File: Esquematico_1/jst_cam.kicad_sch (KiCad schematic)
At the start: 19 parts, among them J1 Screw_Terminal_01x04, J2 Screw_Terminal_01x03, J3 Screw_Terminal_01x06, J4 Screw_Terminal_01x08, J5 SWD, J6 Screw_Terminal_01x04, J7 USB_C_Receptacle_USB2.0_16P, J8 Screw_Terminal_01x01, J9 Screw_Terminal_01x01, U5 USBLC6-2SC6

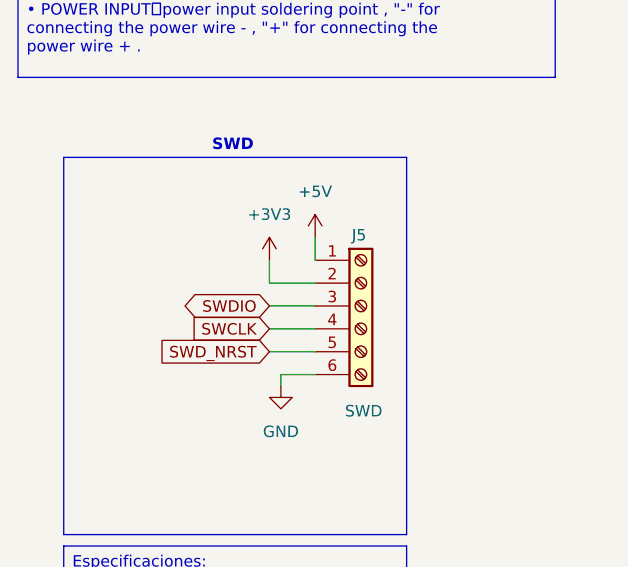
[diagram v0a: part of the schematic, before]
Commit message: Cambios de Diodos
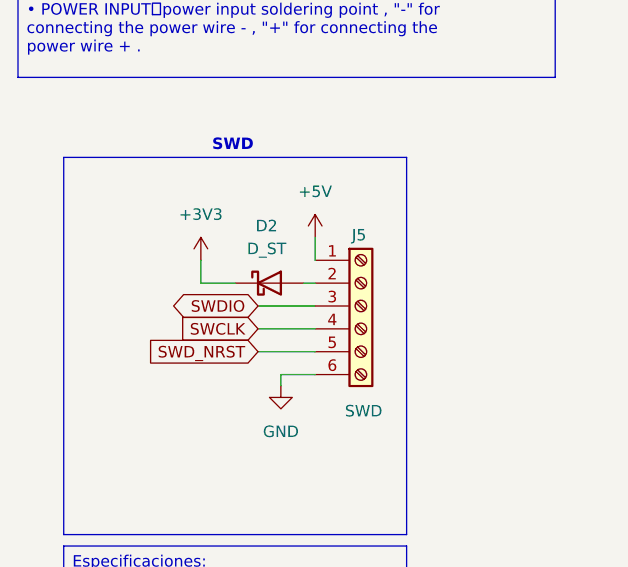
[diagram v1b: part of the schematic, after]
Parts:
- added D2: D_ST, Diode_SMD:D_SOD-323_HandSoldering, symbol Device:D_Schottky
- D3: footprint Package_TO_SOT_SMD:SOT-23 -> Diode_SMD:D_SOD-323_HandSoldering
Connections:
- net +3V3: now also D2.1 (K); no longer J5.2 (Pin_2)
- new net: D2.2 (A), J5.2 (Pin_2)
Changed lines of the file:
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@@
 	(wire
 		(pts
-			(xy 52.07 120.65) (xy 46.99 120.65)
+			(xy 45.72 45.72) (xy 49.53 45.72)
 		)
 		(stroke
@@
 	(wire
 		(pts
-			(xy 45.72 45.72) (xy 49.53 45.72)
+			(xy 63.5 40.64) (xy 68.58 40.64)
 		)
 		(stroke
@@
 	(wire
 		(pts
-			(xy 63.5 40.64) (xy 68.58 40.64)
+			(xy 130.81 133.35) (xy 130.81 130.81)
 		)
 		(stroke
@@
 	(wire
 		(pts
-			(xy 130.81 133.35) (xy 130.81 130.81)
+			(xy 127 50.8) (xy 127 54.61)
 		)
 		(stroke
@@
 	(wire
 		(pts
-			(xy 127 50.8) (xy 127 54.61)
+			(xy 39.37 120.65) (xy 39.37 118.11)
 		)
 		(stroke
@@
 	(wire
 		(pts
-			(xy 46.99 120.65) (xy 46.99 118.11)
+			(xy 50.8 120.65) (xy 52.07 120.65)
 		)
 		(stroke
@@
 	(wire
 		(pts
-			(xy 46.99 123.19) (xy 52.07 123.19)
+			(xy 45.72 123.19) (xy 52.07 123.19)
 		)
 		(stroke
@@
 	(wire
 		(pts
-			(xy 46.99 128.27) (xy 52.07 128.27)
+			(xy 45.72 128.27) (xy 52.07 128.27)
 		)
 		(stroke
@@
 	(wire
 		(pts
-			(xy 46.99 125.73) (xy 52.07 125.73)
+			(xy 45.72 125.73) (xy 52.07 125.73)
 		)
 		(stroke
@@
 	(wire
 		(pts
+			(xy 39.37 120.65) (xy 43.18 120.65)
+		)
+		(stroke
+			(width 0)
+			(type default)
+		)
+	)
+	(wire
+		(pts
 			(xy 139.7 137.16) (xy 139.7 135.89)
 		)
@@
 	(global_label "SWD_NRST"
 		(shape input)
-		(at 46.99 128.27 180)
+		(at 45.72 128.27 180)
 		(fields_autoplaced yes)
 		(effects
@@
 		)
 		(property "Intersheetrefs" "${INTERSHEET_REFS}"
-			(at 34.3287 128.27 0)
+			(at 33.0587 128.27 0)
 			(effects
 				(font
@@
 	(global_label "SWCLK"
 		(shape input)
-		(at 46.99 125.73 180)
+		(at 45.72 125.73 180)
 		(fields_autoplaced yes)
 		(effects
@@
 		)
 		(property "Intersheetrefs" "${INTERSHEET_REFS}"
-			(at 37.7758 125.73 0)
+			(at 36.5058 125.73 0)
 			(effects
 				(font
@@
 	(global_label "SWDIO"
 		(shape bidirectional)
-		(at 46.99 123.19 180)
+		(at 45.72 123.19 180)
 		(fields_autoplaced yes)
 		(effects
@@
 		)
 		(property "Intersheetrefs" "${INTERSHEET_REFS}"
-			(at 37.0273 123.19 0)
+			(at 35.7573 123.19 0)
 			(effects
 				(font
@@
 	(symbol
 		(lib_id "power:+3V3")
-		(at 46.99 118.11 0)
+		(at 39.37 118.11 0)
 		(unit 1)
 		(exclude_from_sim no)
@@
 		(fields_autoplaced yes)
 		(property "Reference" "#PWR037"
-			(at 46.99 121.92 0)
+			(at 39.37 121.92 0)
 			(effects
 				(font
@@
 		)
 		(property "Value" "+3V3"
-			(at 46.99 113.03 0)
+			(at 39.37 113.03 0)
 			(effects
 				(font
@@
 		)
 		(property "Footprint" ""
-			(at 46.99 118.11 0)
+			(at 39.37 118.11 0)
 			(effects
 				(font
@@
 		)
 		(property "Datasheet" ""
-			(at 46.99 118.11 0)
+			(at 39.37 118.11 0)
 			(effects
 				(font
@@
 		)
 		(property "Description" "Power symbol creates a global label with name \"+3V3\""
-			(at 46.99 118.11 0)
+			(at 39.37 118.11 0)
 			(effects
 				(font
@@
 			)
 		)
-		(property "Footprint" "Package_TO_SOT_SMD:SOT-23"
+		(property "Footprint" "Diode_SMD:D_SOD-323_HandSoldering"
 			(at 133.35 113.03 0)
 			(effects
@@
 					(unit 1)
 				)
+			)
+		)
+	)
+	(symbol
+		(lib_id "Device:D_Schottky")
+		(at 46.99 120.65 0)
+		(unit 1)
+		(exclude_from_sim no)
+		(in_bom yes)
+		(on_board yes)
+		(dnp no)
+		(fields_autoplaced yes)
+		(property "Reference" "D2"
+			(at 46.6725 114.3 0)
+			(effects
+				(font
+					(size 1.27 1.27)
+				)
+			)
+		)
+		(property "Value" "D_ST"
+			(at 46.6725 116.84 0)
+			(effects
+				(font
+					(size 1.27 1.27)
+				)
+			)
+		)
+		(property "Footprint" "Diode_SMD:D_SOD-323_HandSoldering"
+			(at 46.99 120.65 0)
+			(effects
+				(font
+					(size 1.27 1.27)
+				)
+				(hide yes)
+			)
+		)
+		(property "Datasheet" "~"
+			(at 46.99 120.65 0)
+			(effects
+				(font
+					(size 1.27 1.27)
+				)
+				(hide yes)
+			)
+		)
+		(property "Description" "Schottky diode"
+			(at 46.99 120.65 0)
+			(effects
+				(font
+					(size 1.27 1.27)
+				)
+				(hide yes)
+			)
+		)
+		(pin "1"
+		)
+		(pin "2"
+		)
+		(instances
+			(project "Esquematico_1"
+				(path "/de2d80c1-c21c-478d-b724-17659b714c38/457e76de-adfe-4ec5-a818-c5970caa89a7"
+					(reference "D2")
+					(unit 1)
+				)
